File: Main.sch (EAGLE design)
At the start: 29 parts, among them Q1 IRF9530, U1 L298, U2 LM 1084 IT5,0, U3 LM 1084 IT3,3, U4 L298, X1 Motors, X2 PIRs, X3 Battery

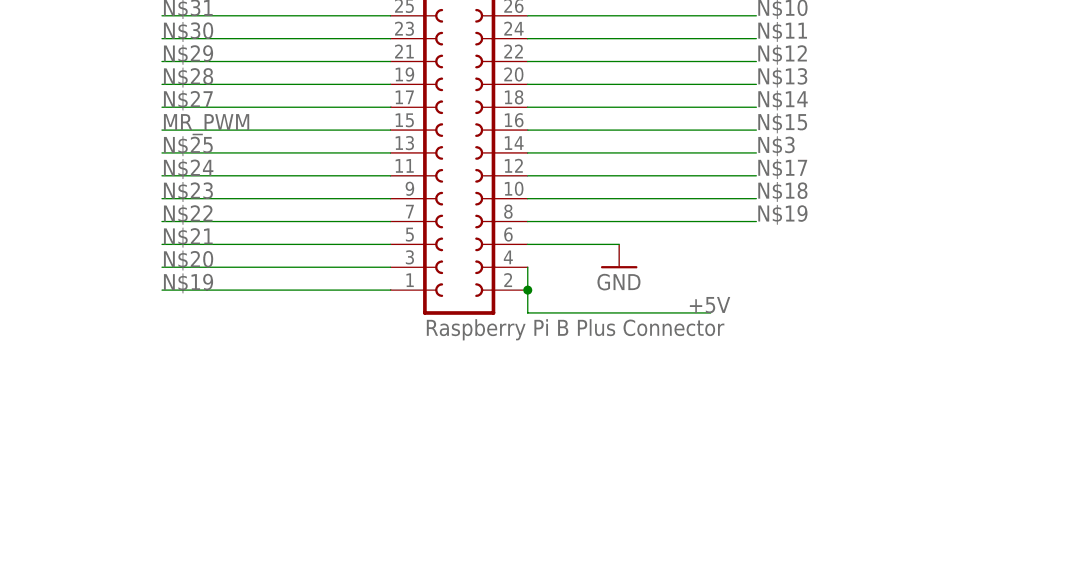
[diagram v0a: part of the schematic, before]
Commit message: some cleanup
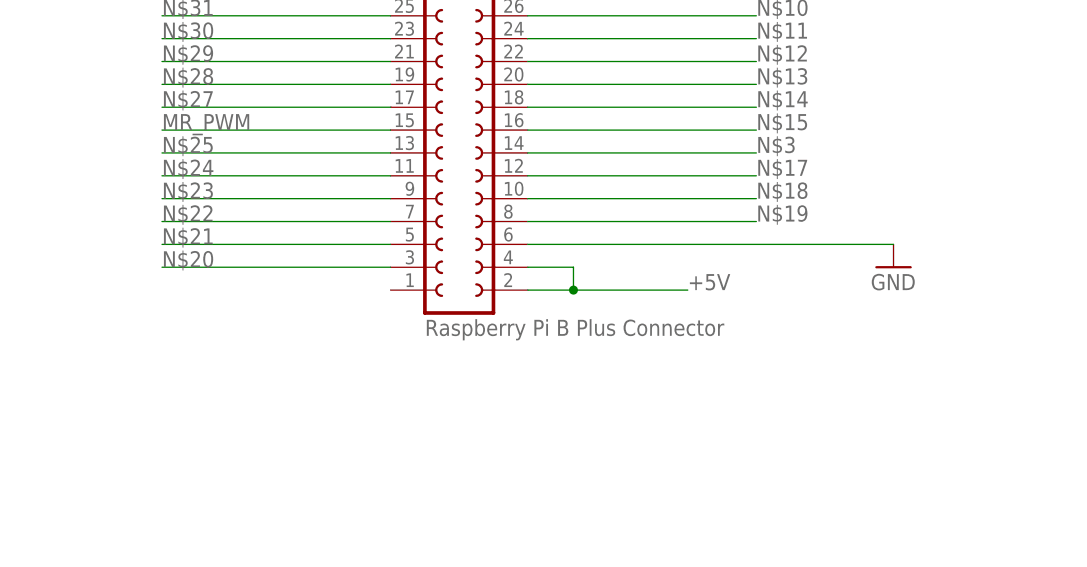
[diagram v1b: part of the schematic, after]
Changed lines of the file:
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@@
 <instance part="GND3" gate="1" x="-487.68" y="137.16"/>
 <instance part="SV1" gate="G$1" x="-388.62" y="518.16"/>
-<instance part="GND4" gate="1" x="-370.84" y="495.3"/>
+<instance part="GND4" gate="1" x="-340.36" y="495.3"/>
 <instance part="D2" gate="G$1" x="-381" y="167.64" rot="R90"/>
 <instance part="D3" gate="G$1" x="-398.78" y="167.64" rot="R90"/>
@@
 </segment>
 <segment>
+<pinref part="SV1" gate="G$1" pin="2"/>
+<wire x1="-381" y1="492.76" x2="-375.92" y2="492.76" width="0.1524" layer="91"/>
+<wire x1="-363.22" y1="492.76" x2="-375.92" y2="492.76" width="0.1524" layer="91"/>
+<wire x1="-375.92" y1="492.76" x2="-375.92" y2="495.3" width="0.1524" layer="91"/>
+<junction x="-375.92" y="492.76"/>
 <pinref part="SV1" gate="G$1" pin="4"/>
-<pinref part="SV1" gate="G$1" pin="2"/>
-<wire x1="-381" y1="495.3" x2="-381" y2="492.76" width="0.1524" layer="91"/>
-<wire x1="-381" y1="492.76" x2="-381" y2="490.22" width="0.1524" layer="91"/>
-<junction x="-381" y="492.76"/>
-<wire x1="-381" y1="490.22" x2="-360.68" y2="490.22" width="0.1524" layer="91"/>
-<label x="-363.22" y="490.22" size="1.778" layer="95"/>
+<wire x1="-375.92" y1="495.3" x2="-381" y2="495.3" width="0.1524" layer="91"/>
+<label x="-363.22" y="492.76" size="1.778" layer="95"/>
 </segment>
 </net>
@@
 <pinref part="SV1" gate="G$1" pin="6"/>
 <pinref part="GND4" gate="1" pin="GND"/>
-<wire x1="-381" y1="497.84" x2="-370.84" y2="497.84" width="0.1524" layer="91"/>
+<wire x1="-381" y1="497.84" x2="-340.36" y2="497.84" width="0.1524" layer="91"/>
 </segment>
 <segment>
@@
 <label x="-355.6" y="500.38" size="1.778" layer="95"/>
 </segment>
-<segment>
-<wire x1="-421.64" y1="492.76" x2="-396.24" y2="492.76" width="0.1524" layer="91"/>
-<label x="-421.64" y="492.76" size="1.778" layer="95"/>
-</segment>
-</net>
+</net>

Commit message: fuses
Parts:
- removed C3: 10uF Tant., rcl:C-EU025-040X050
- added F1: PFRA 600, Sicherungselemente:PTC-SICHERUNG-2.50
- added F2: PTC194600-110, _hhn_PtcFuses_Siba_r500:SIBA194600
- added F3, F4, F5, F6: PTC194600-150, _hhn_PtcFuses_Siba_r500:SIBA194600
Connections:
- new net N$26: F4.2, X1-3.1
- new net N$34: F5.2, X1-5.1
- new net N$36: F6.2, X1-7.1
- new net N$4: F1.1, X3-1.1
- new net N$5: F2.1, SV1.2, SV1.4
- new net N$7: F3.2, X1-1.1
- net +12V: no longer C3.1
- net +5V: now also F2.2; no longer SV1.2, SV1.4
- net GND: no longer C3.2
- net ML_OUT_A: now also F3.1, F4.1; no longer X1-1.1, X1-3.1
- net MR_OUT_A: now also F5.1, F6.1; no longer X1-5.1, X1-7.1
- net N$1: now also F1.2; no longer X3-1.1
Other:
- moved on the sheet: C1, C2, C4, D1, D5, D6, Q1, R1, U2, U3, X1-1, X1-2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
